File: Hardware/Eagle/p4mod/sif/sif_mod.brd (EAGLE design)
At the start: 19.6 x 10.8 mm, 29 parts

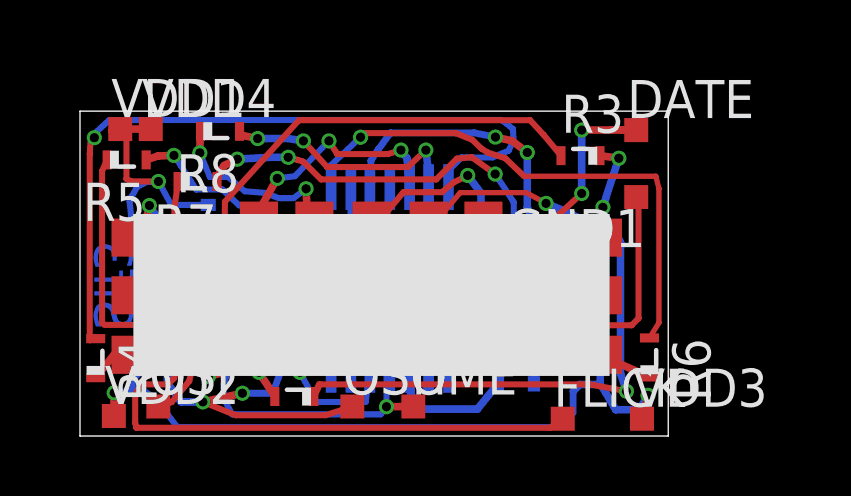
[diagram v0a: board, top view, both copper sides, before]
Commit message: Optimizations.
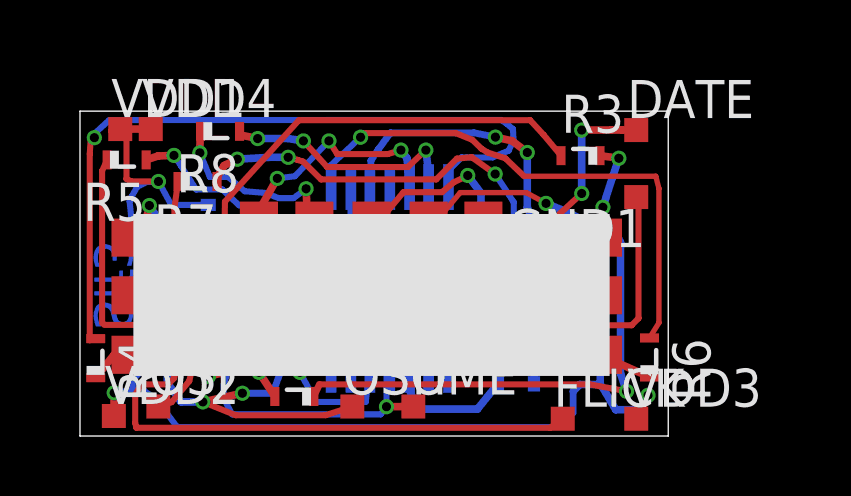
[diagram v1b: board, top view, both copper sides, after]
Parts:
- moved VDD3 0.19 mm to (19.8, 0.75)
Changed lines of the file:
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@@
 <attribute name="TP_SIGNAL_NAME" value="" x="2.34269375" y="0.836640625" size="1.778" layer="27" display="off"/>
 </element>
-<element name="VDD3" library="testpad" package="TP08SQ" value="TPTP08SQ" x="19.94685625" y="0.745434375">
-<attribute name="TP_SIGNAL_NAME" value="" x="19.94685625" y="0.745434375" size="1.778" layer="27" display="off"/>
+<element name="VDD3" library="testpad" package="TP08SQ" value="TPTP08SQ" x="19.754278125" y="0.745434375">
+<attribute name="TP_SIGNAL_NAME" value="" x="19.754278125" y="0.745434375" size="1.778" layer="27" display="off"/>
 </element>
 <element name="VDD1" library="testpad" package="TP08SQ" value="TPTP08SQ" x="2.554646875" y="10.4011125">
@@
 <wire x1="18.6182" y1="1.8143125" x2="18.55316875" y2="1.88485625" width="0.1524" layer="16"/>
 <via x="20.148546875" y="1.526584375" extent="1-16" drill="0.3048"/>
-<wire x1="20.148546875" y1="1.526584375" x2="19.94685625" y2="0.745434375" width="0.254" layer="1"/>
+<wire x1="20.148546875" y1="1.526584375" x2="19.754278125" y2="0.745434375" width="0.254" layer="1"/>
 <wire x1="2.92190625" y1="8.65561875" x2="3.82825625" y2="8.65421875" width="0.2032" layer="1"/>
 <wire x1="3.82825625" y1="8.65421875" x2="4.256571875" y2="7.87175" width="0.2032" layer="16"/>
